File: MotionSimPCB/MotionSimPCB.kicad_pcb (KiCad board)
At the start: 2 copper layers, 56 x 70 mm, 55 parts, among them J1 Conn_01x02, J10 Conn_01x02, J11 Raspberry_Pi_4, J12 AudioJack2, J13 Conn_01x03, J14 Conn_01x03, J2 Conn_01x08_Pin, J3 Conn_01x03, J4 Conn_01x03, J5 Conn_01x03, J6 Conn_01x03, J7 Conn_01x02, J8 Conn_01x02, J9 Conn_01x02, Q1 BSS138, Q2 IRF7404, U1 MPU-6050, U2 Teensy4.0

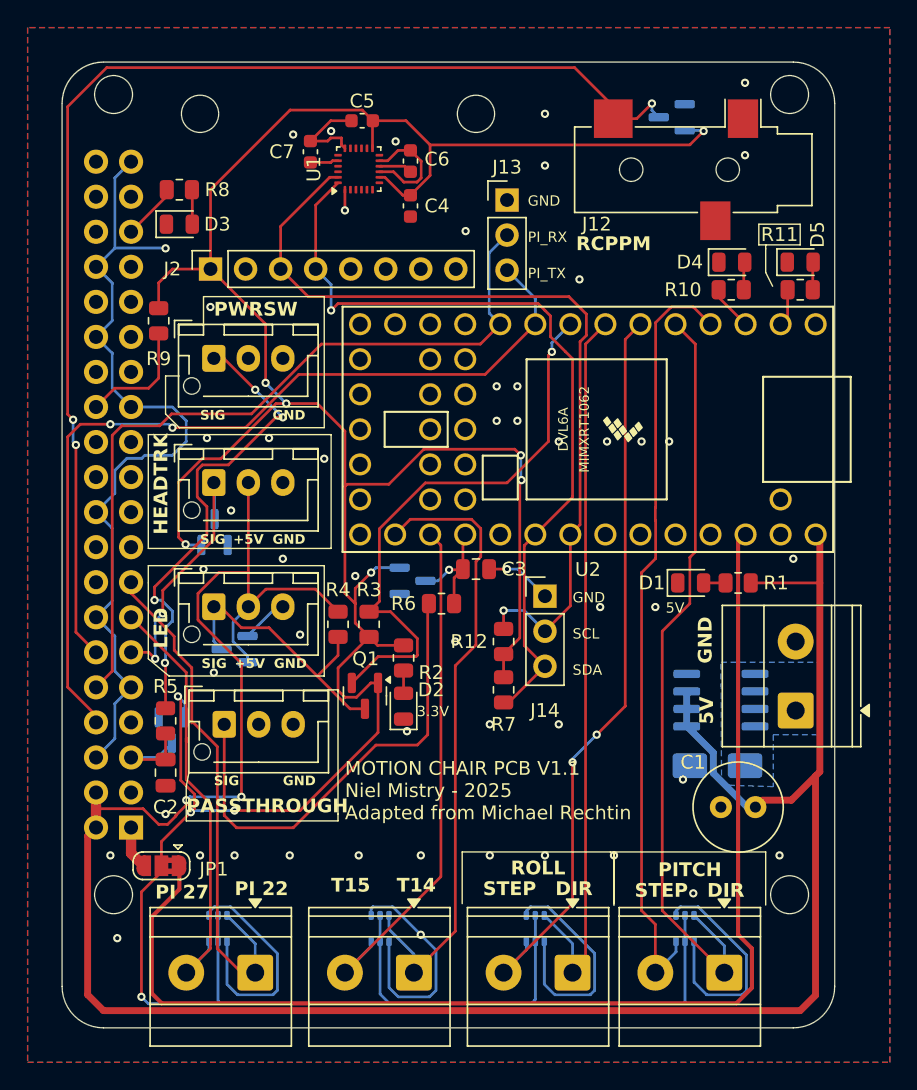
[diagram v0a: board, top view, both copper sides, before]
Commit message: fix some issues
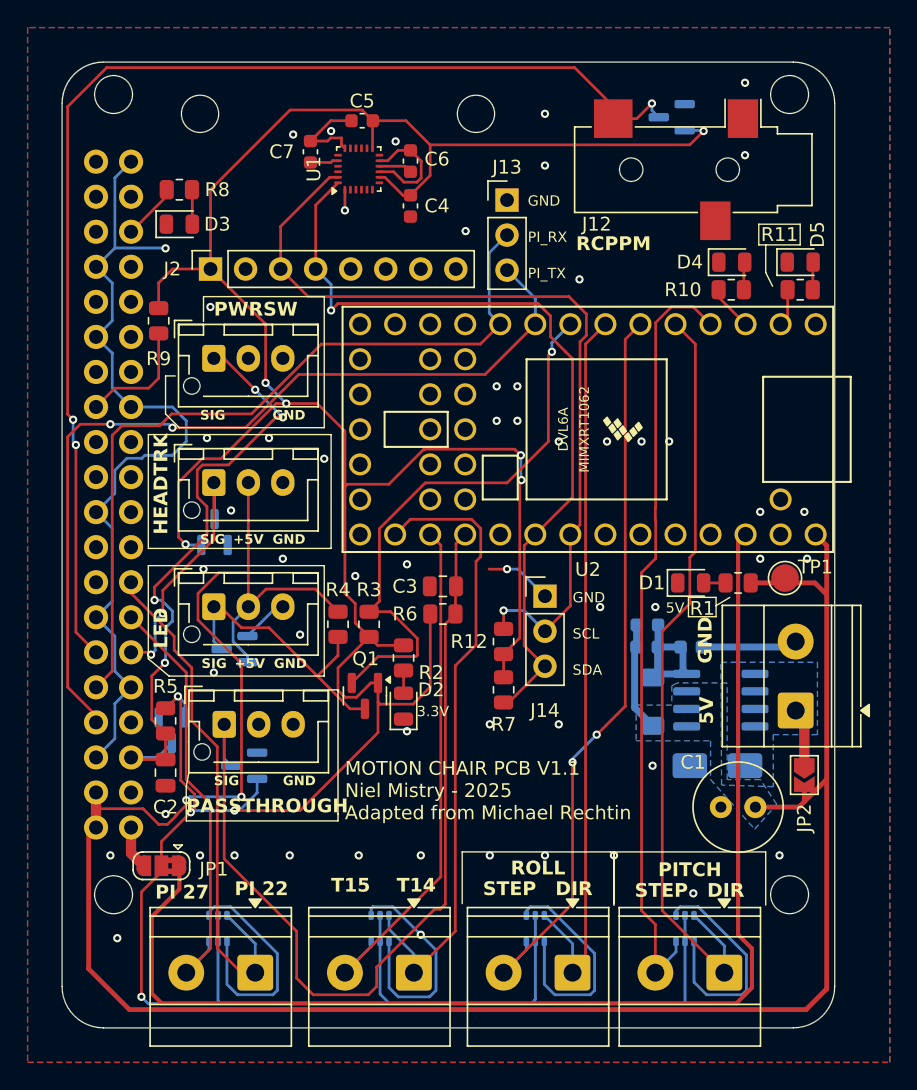
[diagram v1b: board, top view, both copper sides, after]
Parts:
- added C8: 0.1u, Capacitor_SMD:C_0603_1608Metric, B.Cu at (142.4, 80.8)
- added D16: BZV55C12, Diode_SMD:D_MiniMELF, B.Cu at (142.8, 86.3)
- added JP2: SolderJumper_2_Open, Jumper:SolderJumper-2_P1.3mm_Open_TrianglePad1.0x1.5mm, F.Cu at (153.8, 91.7)
- added R13: 100, Capacitor_SMD:C_0603_1608Metric, B.Cu at (145.6, 82.4)
- added R14: 100k, Capacitor_SMD:C_0603_1608Metric, B.Cu at (142.4, 82.4)
- added TP1: TestPoint_Flag, TestPoint:TestPoint_Pad_D2.0mm, F.Cu at (152.4, 77.4)
- moved D13 18.1 mm to (113.2, 91.0), turned to 180 degrees
- moved C3 2.71 mm to (127.6, 78.0), turned to 180 degrees
- moved R6 0.76 mm to (127.6, 80.0)
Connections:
- J3 pad 1: Net-(J3-Pin_1) -> /PWR_OFF_SW
- J4 pad 1: Net-(J4-Pin_1) -> /PASSTHRU
- Q2 pad 4: GND -> Net-(D16-A)
- R5 pad 1: Net-(J3-Pin_1) -> +3.3V
- R6 pad 1: Net-(J4-Pin_1) -> +3.3V
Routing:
- net /PASSTHRU: track 8.41 -> 66.0 mm, vias 1 -> 0
- net /PWR_OFF_SW: track 7.82 -> 45.3 mm, vias 0 -> 4
- net Net-(J3-Pin_1): track 34.8 -> 0.00 mm, vias 4 -> 0
- net Net-(J4-Pin_1): track 34.1 -> 0.00 mm
- net Net-(D16-A): track 0.00 -> 10.3 mm
- net +3.3V: track 268.8 -> 278.0 mm, vias 11 -> 10
- net GND: track 153.5 -> 160.1 mm, vias 52 -> 55
- net Net-(D6-A1): track 0.00 -> 4.21 mm
- net /HEAD_TRK: track 19.2 -> 18.6 mm
- added copper zone on B.Cu, net +5V
